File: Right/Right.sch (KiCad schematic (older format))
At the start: 105 parts, among them SW1 SW_PUSH, SW10 SW_PUSH, SW100 SW_Push_Dual_R, SW101 SW_Push_Dual_R, SW102 SW_Push_Dual_R, SW11 SW_PUSH, SW12 SW_PUSH, SW13 SW_PUSH, SW14 SW_PUSH, SW15 SW_PUSH, SW16 SW_PUSH, SW17 SW_PUSH, SW18 SW_PUSH, SW19 SW_PUSH, SW2 SW_PUSH, SW20 SW_PUSH, SW200 SW_SPDT, SW21 SW_PUSH, SW22 SW_PUSH, SW23 SW_PUSH, SW24 SW_PUSH, SW25 SW_PUSH, SW26 SW_PUSH, SW27 SW_PUSH, SW28 SW_PUSH, SW29 SW_PUSH, SW3 SW_PUSH, SW30 SW_PUSH, SW31 SW_PUSH, SW32 SW_PUSH, SW33 SW_PUSH, SW34 SW_PUSH, SW35 SW_PUSH, SW36 SW_PUSH, SW37 SW_PUSH, SW38 SW_PUSH, SW39 SW_PUSH, SW4 SW_PUSH, SW40 SW_PUSH, SW41 SW_PUSH, SW42 SW_PUSH, SW43 SW_PUSH, SW44 SW_PUSH, SW45 SW_PUSH, SW5 SW_PUSH, SW6 SW_PUSH, SW7 SW_PUSH, SW8 SW_PUSH, SW9 SW_PUSH, U1 CH25-2032LF, U2 CH25-2032LF

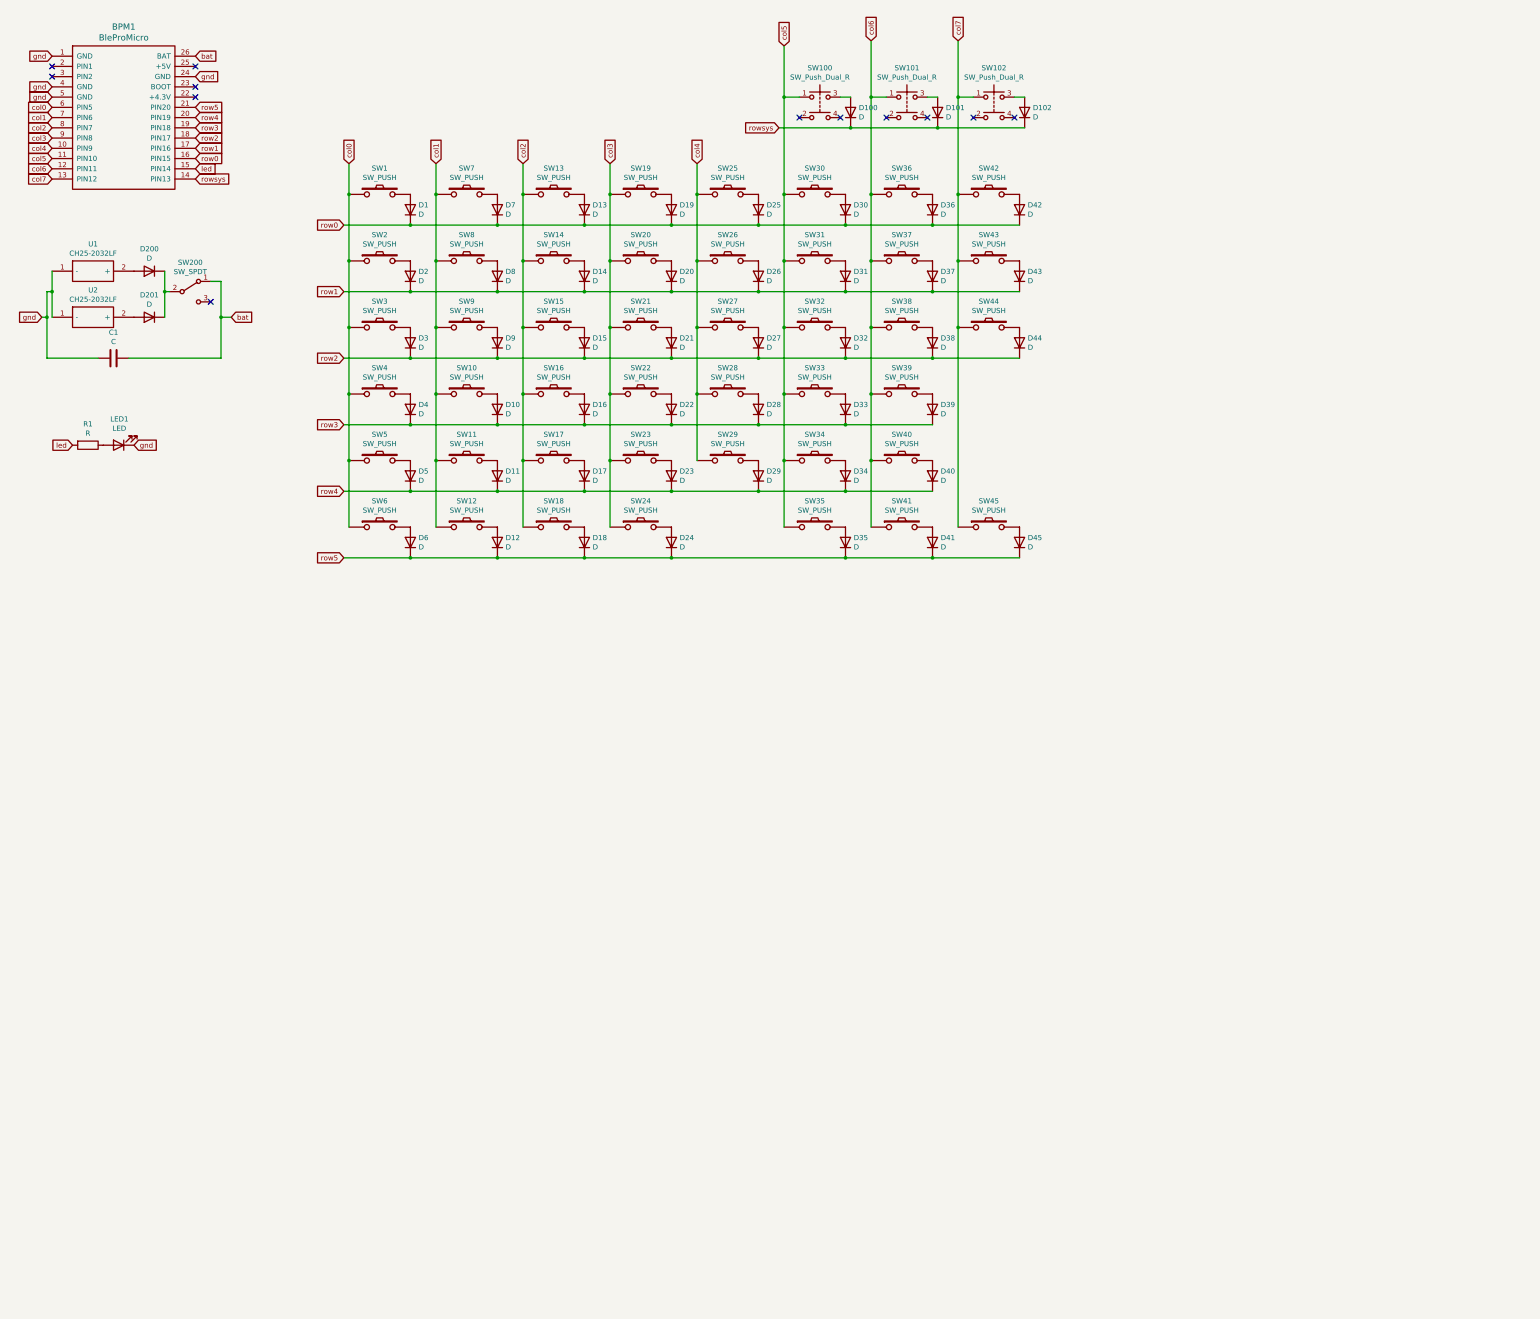
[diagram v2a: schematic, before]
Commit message: 全体にした
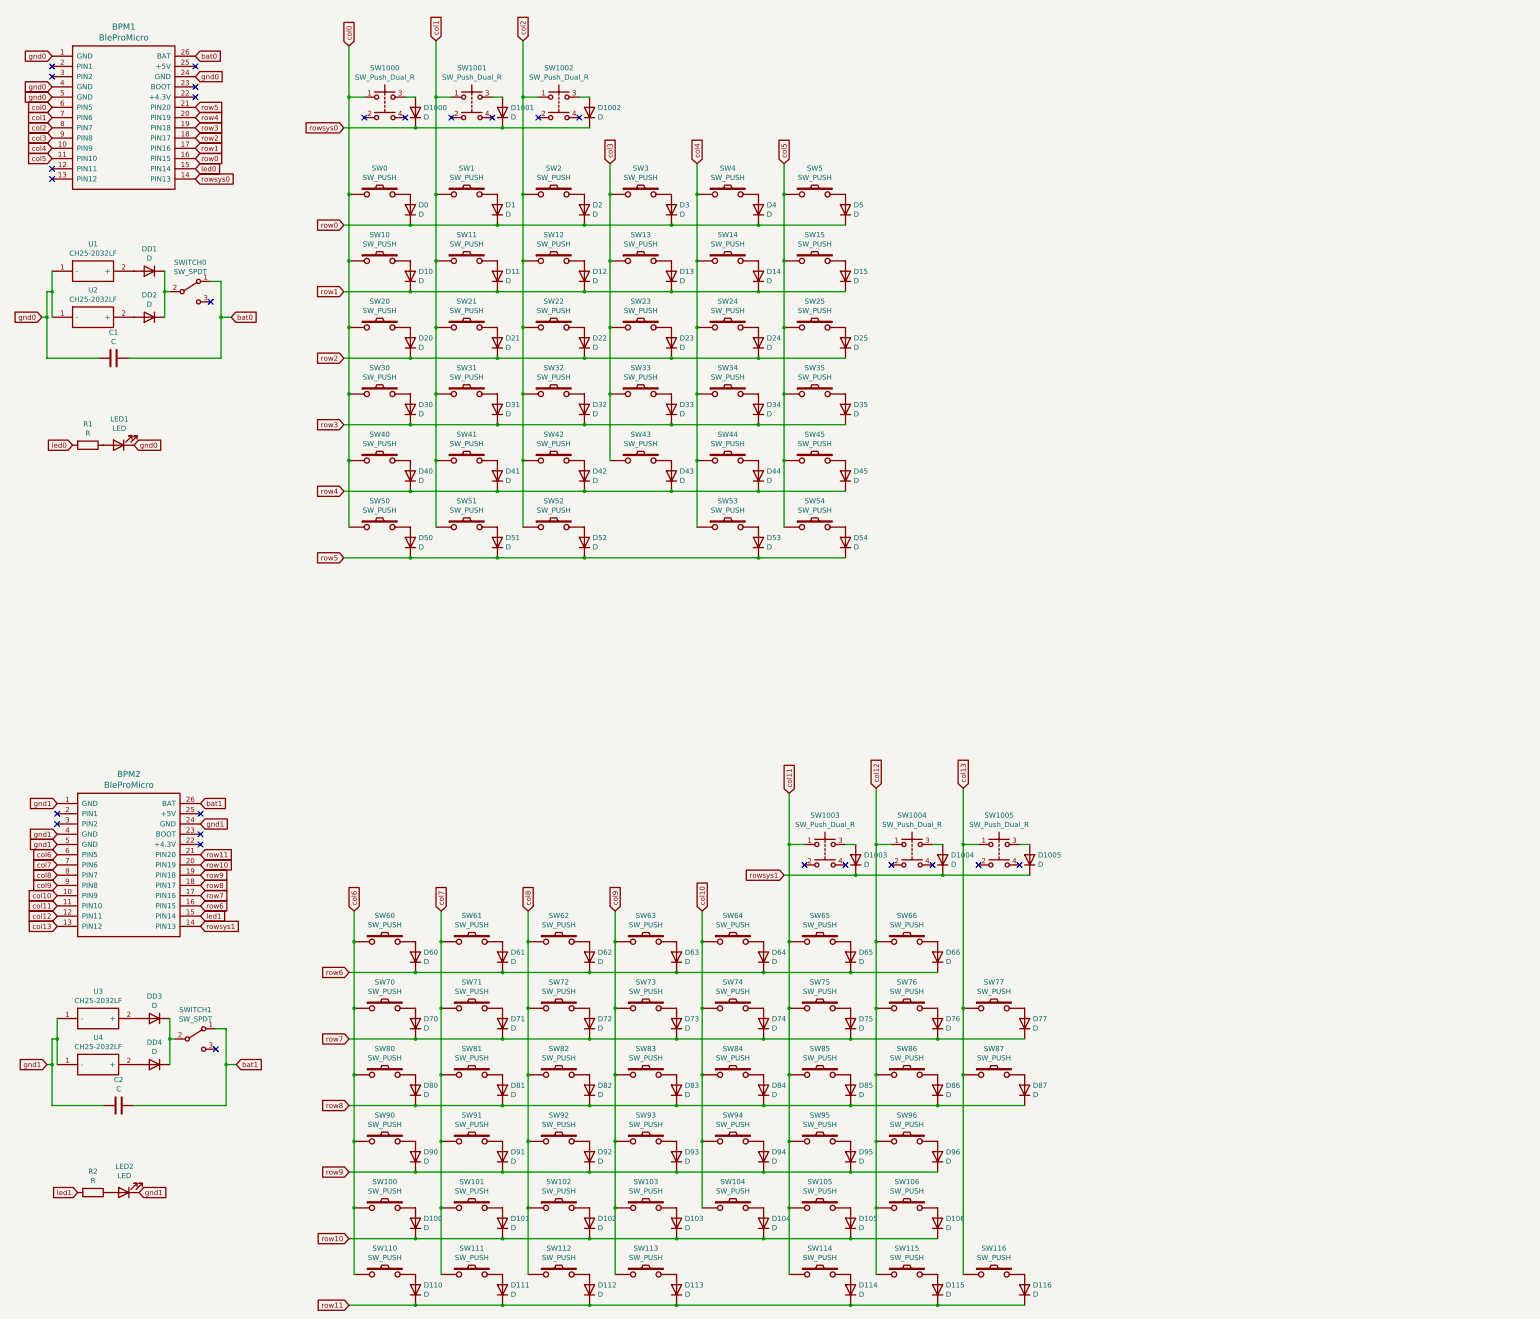
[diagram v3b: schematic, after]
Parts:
- removed D36, D37, D38, D39, D40, D41, D42, D43, D44, D45: D, Diode_THT:D_DO-35_SOD27_P7.62mm_Horizontal, symbol Device:D
- removed SW36, SW37, SW38, SW39, SW40, SW41, SW42, SW43, SW44, SW45: SW_PUSH, keyswitches:Kailh_socket_MX, symbol kbd:SW_PUSH
- added BPM2: BleProMicro, mylibrary:BLEMicroPro, symbol My_Library:BleProMicro
- added C2: C, Capacitor_THT:C_Disc_D5.1mm_W3.2mm_P5.00mm, symbol Device:C
- added D100, D1003, D1004, D1005, D101, D102, D103, D104, D105, D106, D110, D111, D112, D113, D114, D115, D116, D60, D61, D62, D63, D64, D65, D66, D70, D71, D72, D73, D74, D75, D76, D77, D80, D81, D82, D83, D84, D85, D86, D87, D90, D91, D92, D93, D94, D95, D96: D, Diode_THT:D_DO-35_SOD27_P7.62mm_Horizontal, symbol Device:D
- added DD3, DD4: D, Diode_THT:D_DO-41_SOD81_P7.62mm_Horizontal, symbol Device:D
- added LED2: LED, LED_THT:LED_D3.0mm, symbol Device:LED
- added R2: R, Resistor_THT:R_Axial_DIN0204_L3.6mm_D1.6mm_P7.62mm_Horizontal, symbol Device:R
- added SW100, SW101, SW102, SW103, SW104, SW105, SW106, SW110, SW111, SW112, SW113, SW114, SW115, SW116, SW60, SW61, SW62, SW63, SW64, SW65, SW66, SW70, SW71, SW72, SW73, SW74, SW75, SW76, SW77, SW80, SW81, SW82, SW83, SW84, SW85, SW86, SW87, SW90, SW91, SW92, SW93, SW94, SW95, SW96: SW_PUSH, keyswitches:Kailh_socket_MX, symbol kbd:SW_PUSH
- added SW1003, SW1004, SW1005: SW_Push_Dual_R, Button_Switch_THT:SW_TH_Tactile_Omron_B3F-10xx, symbol My_Library:SW_Push_Dual_R
- added SWITCH1: SW_SPDT, mylibrary:2MS1-T1-B4-VS2-Q-E-S, symbol Switch:SW_SPDT
- added U3, U4: CH25-2032LF, CH25-2032LF:CH252032LF, symbol CH25-2032LF:CH25-2032LF
- renumbered D1 to D0, D7 to D1, D2 to D10, D100 to D1000, D101 to D1001, D102 to D1002, D8 to D11, D14 to D12, D20 to D13, D26 to D14, D31 to D15, D13 to D2, D3 to D20, D9 to D21, D15 to D22, D21 to D23, D27 to D24, D32 to D25, D19 to D3, D4 to D30, D10 to D31, D16 to D32, D22 to D33, D28 to D34, D33 to D35, D25 to D4, D5 to D40, D11 to D41, D17 to D42, D23 to D43, D29 to D44, D34 to D45, D30 to D5, D6 to D50, D12 to D51, D18 to D52, D24 to D53, D35 to D54, D200 to DD1, D201 to DD2, SW1 to SW0, SW7 to SW1, SW2 to SW10, SW100 to SW1000, SW101 to SW1001, SW102 to SW1002, SW8 to SW11, SW14 to SW12, SW20 to SW13, SW26 to SW14, SW31 to SW15, SW13 to SW2, SW3 to SW20, SW9 to SW21, SW15 to SW22, SW21 to SW23, SW27 to SW24, SW32 to SW25, SW19 to SW3, SW4 to SW30, SW10 to SW31, SW16 to SW32, SW22 to SW33, SW28 to SW34, SW33 to SW35, SW25 to SW4, SW5 to SW40, SW11 to SW41, SW17 to SW42, SW23 to SW43, SW29 to SW44, SW34 to SW45, SW30 to SW5, SW6 to SW50, SW12 to SW51, SW18 to SW52, SW24 to SW53, SW35 to SW54, SW200 to SWITCH0
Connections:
- net col0: now also SW1000.1
- net col1: now also SW1001.1
- net col2: now also SW1002.1
- net col3: no longer SW53.1
- net col4: now also SW53.1
- net col5: no longer SW1000.1
- net col6: now also BPM2.6 (PIN5), SW100.1, SW110.1, SW60.1, SW70.1, SW80.1, SW90.1; no longer BPM1.12 (PIN11), SW1001.1
- net col7: now also BPM2.7 (PIN6), SW101.1, SW111.1, SW61.1, SW71.1, SW81.1, SW91.1; no longer BPM1.13 (PIN12), SW1002.1
- net bat renamed bat0
- net gnd renamed gnd0
- net led renamed led0
- net rowsys renamed rowsys0
- new net: D61.2 (A), SW61.2
- new net: D60.2 (A), SW60.2
- new net: D62.2 (A), SW62.2
- new net: D63.2 (A), SW63.2
- new net: D65.2 (A), SW65.2
- new net: D64.2 (A), SW64.2
- new net: D66.2 (A), SW66.2
- new net: D71.2 (A), SW71.2
- new net: D70.2 (A), SW70.2
- new net: D72.2 (A), SW72.2
- new net: D73.2 (A), SW73.2
- new net: D75.2 (A), SW75.2
- new net: D74.2 (A), SW74.2
- new net: D76.2 (A), SW76.2
- new net: D77.2 (A), SW77.2
- new net: D81.2 (A), SW81.2
- new net: D80.2 (A), SW80.2
- new net: D82.2 (A), SW82.2
- new net: D83.2 (A), SW83.2
- new net: D85.2 (A), SW85.2
- new net: D84.2 (A), SW84.2
- new net: D86.2 (A), SW86.2
- new net: D87.2 (A), SW87.2
- new net: D91.2 (A), SW91.2
- new net: D90.2 (A), SW90.2
- new net: D92.2 (A), SW92.2
- new net: D93.2 (A), SW93.2
- new net: D95.2 (A), SW95.2
- new net: D94.2 (A), SW94.2
- new net: D96.2 (A), SW96.2
- new net: D101.2 (A), SW101.2
- new net: D100.2 (A), SW100.2
- new net: D102.2 (A), SW102.2
- new net: D103.2 (A), SW103.2
- new net: D105.2 (A), SW105.2
- new net: D104.2 (A), SW104.2
- new net: D106.2 (A), SW106.2
- new net: D111.2 (A), SW111.2
- new net: D110.2 (A), SW110.2
- new net: D112.2 (A), SW112.2
- new net: D113.2 (A), SW113.2
- new net: D114.2 (A), SW114.2
- new net: D115.2 (A), SW115.2
- new net: DD3.2 (A), U3.2 (+)
- new net: DD3.1 (K), DD4.1 (K), SWITCH1.2 (B)
- new net: DD4.2 (A), U4.2 (+)
- new net: LED2.2 (A), R2.1
- new net: D116.2 (A), SW116.2
- new net: D1003.2 (A), SW1003.3
- new net: D1004.2 (A), SW1004.3
- new net: D1005.2 (A), SW1005.3
- new net bat1: BPM2.26 (BAT), C2.1, SWITCH1.1 (A)
- new net col10: BPM2.10 (PIN9), SW104.1, SW64.1, SW74.1, SW84.1, SW94.1
- new net col11: BPM2.11 (PIN10), SW1003.1, SW105.1, SW114.1, SW65.1, SW75.1, SW85.1, SW95.1
- new net col12: BPM2.12 (PIN11), SW1004.1, SW106.1, SW115.1, SW66.1, SW76.1, SW86.1, SW96.1
- new net col13: BPM2.13 (PIN12), SW1005.1, SW116.1, SW77.1, SW87.1
- new net col8: BPM2.8 (PIN7), SW102.1, SW112.1, SW62.1, SW72.1, SW82.1, SW92.1
- new net col9: BPM2.9 (PIN8), SW103.1, SW113.1, SW63.1, SW73.1, SW83.1, SW93.1
- new net gnd1: BPM2.1 (GND), BPM2.24 (GND), BPM2.4 (GND), BPM2.5 (GND), C2.2, LED2.1 (K), U3.1 (-), U4.1 (-)
- new net led1: BPM2.15 (PIN14), R2.2
- new net row10: BPM2.20 (PIN19), D100.1 (K), D101.1 (K), D102.1 (K), D103.1 (K), D104.1 (K), D105.1 (K), D106.1 (K)
- new net row11: BPM2.21 (PIN20), D110.1 (K), D111.1 (K), D112.1 (K), D113.1 (K), D114.1 (K), D115.1 (K), D116.1 (K)
- new net row6: BPM2.16 (PIN15), D60.1 (K), D61.1 (K), D62.1 (K), D63.1 (K), D64.1 (K), D65.1 (K), D66.1 (K)
- new net row7: BPM2.17 (PIN16), D70.1 (K), D71.1 (K), D72.1 (K), D73.1 (K), D74.1 (K), D75.1 (K), D76.1 (K), D77.1 (K)
- new net row8: BPM2.18 (PIN17), D80.1 (K), D81.1 (K), D82.1 (K), D83.1 (K), D84.1 (K), D85.1 (K), D86.1 (K), D87.1 (K)
- new net row9: BPM2.19 (PIN18), D90.1 (K), D91.1 (K), D92.1 (K), D93.1 (K), D94.1 (K), D95.1 (K), D96.1 (K)
- new net rowsys1: BPM2.14 (PIN13), D1003.1 (K), D1004.1 (K), D1005.1 (K)
- no-connect marks 12 -> 26
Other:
- moved on the sheet: D1000, D1001, D1002, D53, SW1000, SW1001, SW1002, SW53

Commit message: 途中
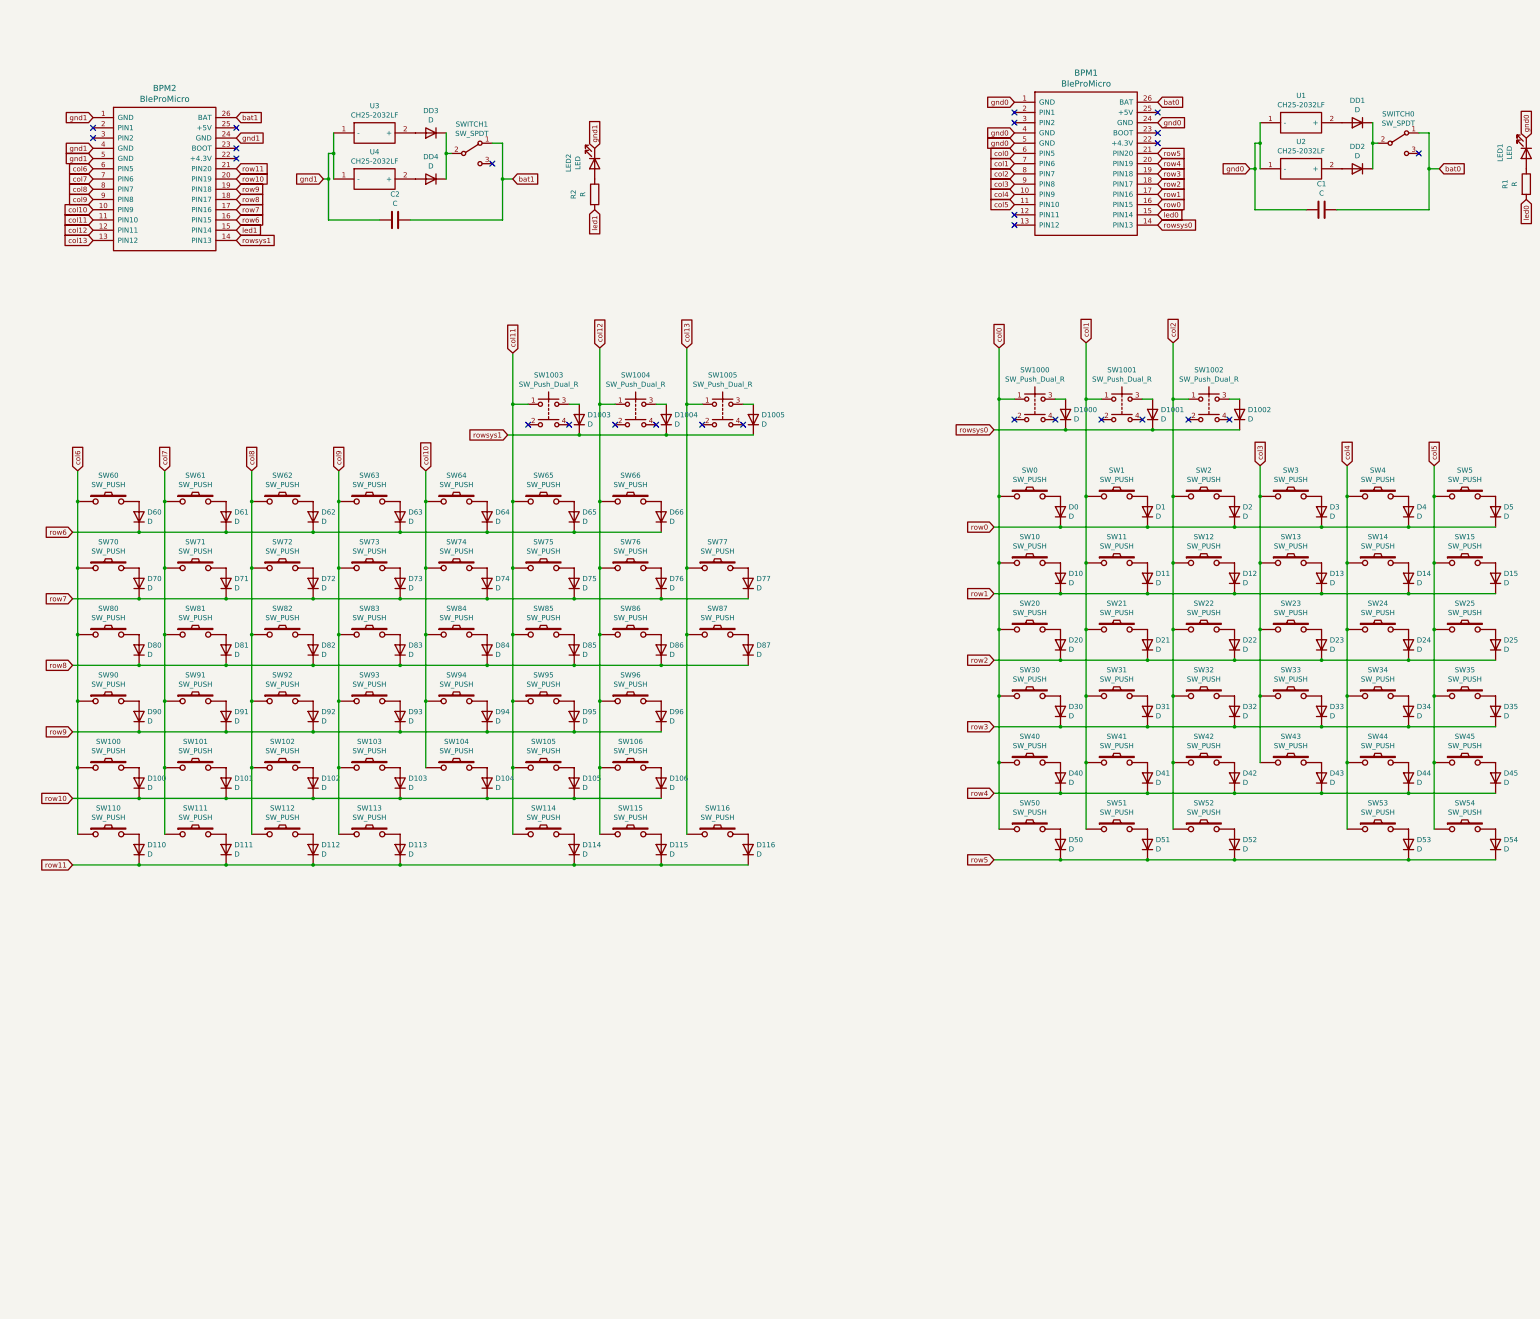
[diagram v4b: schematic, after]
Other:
- moved on the sheet: BPM1, BPM2, C1, C2, D0, D1, D10, D100, D1000, D1001, D1002, D1003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
